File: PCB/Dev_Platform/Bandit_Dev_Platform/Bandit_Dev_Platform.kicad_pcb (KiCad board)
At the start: 4 copper layers, 63.5 x 31.8 mm, 137 parts, among them J12 Conn_01x02_Pin, J5 BNC, J6 BNC, P1 USB_C_Plug_USB2.0, SW1 SW_SPST, U1 AD7253, U10 OPA1664, U11 XC6206PxxxMR, U2 RP2040, U4 NCP164ASNADJT1G, U5 W25Q16JVUXIQ_TR, U6 MCP6486UT-E/OT, U7 MCP6S92-E/SN, U9 OPA1664, Y1 12.000 MHz, C9002

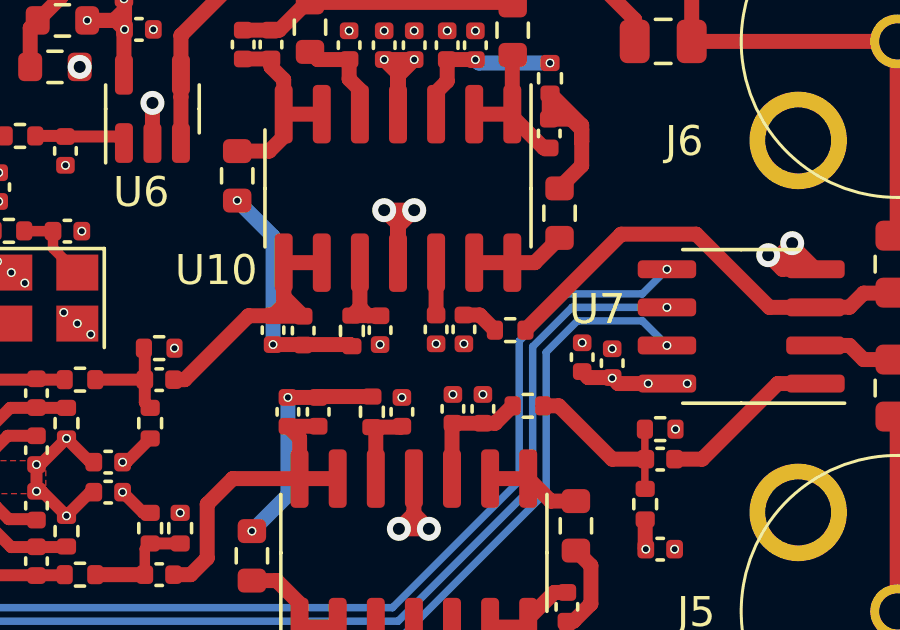
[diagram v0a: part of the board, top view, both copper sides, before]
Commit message: It's workingggggg (mostly)
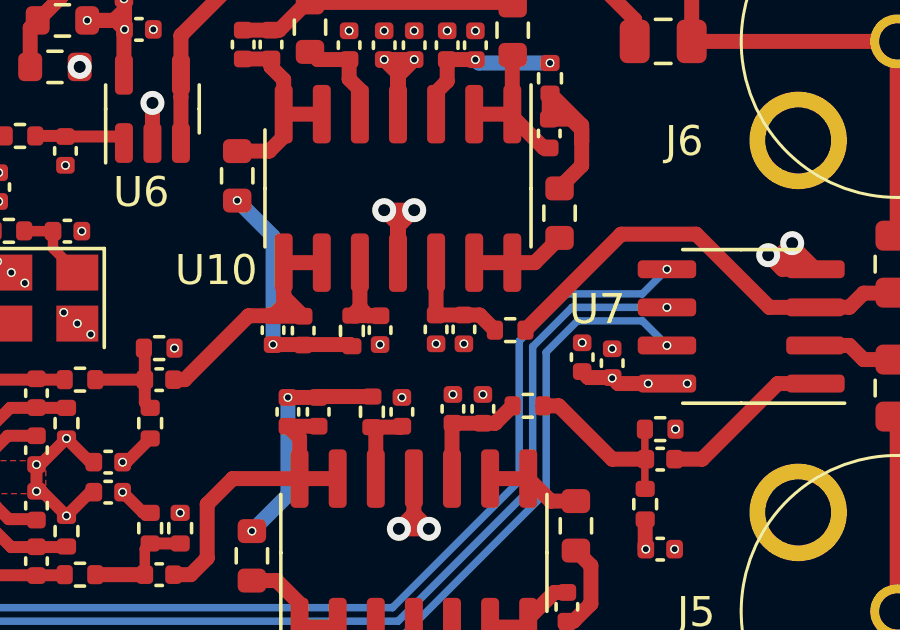
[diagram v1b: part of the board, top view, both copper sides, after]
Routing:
- net Net-(U10D-+): track 2.99 -> 3.91 mm
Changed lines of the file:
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@@
   (segment (start 62.0519 27.0947) (end 64.4273 27.0947) (width 0.5) (layer "B.Cu") (net 18))
   (segment (start 61.9398 26.9826) (end 62.0519 27.0947) (width 0.5) (layer "B.Cu") (net 18))
+  (segment (start 60.63 35.4946) (end 61.5571 35.4946) (width 0.5) (layer "F.Cu") (net 19))
   (segment (start 60.63 33.75) (end 60.63 35.4946) (width 0.5) (layer "F.Cu") (net 19))
   (segment (start 62.59 36) (end 62.0846 35.4946) (width 0.5) (layer "F.Cu") (net 19))
